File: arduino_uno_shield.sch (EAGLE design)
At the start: 13 parts

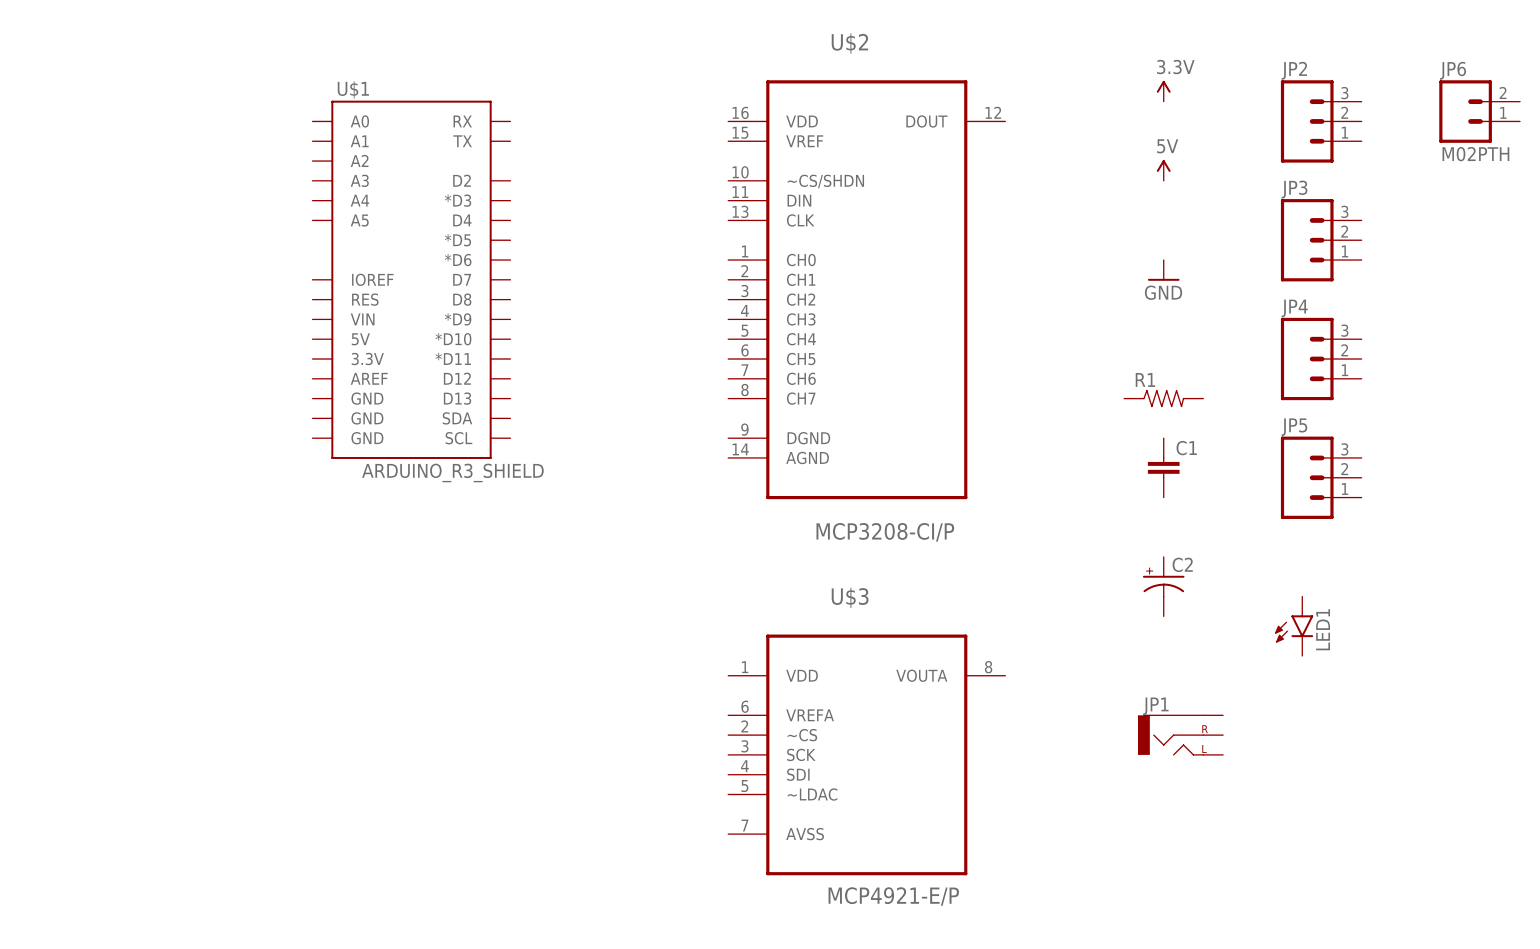
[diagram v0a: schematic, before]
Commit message: wiring up schematic
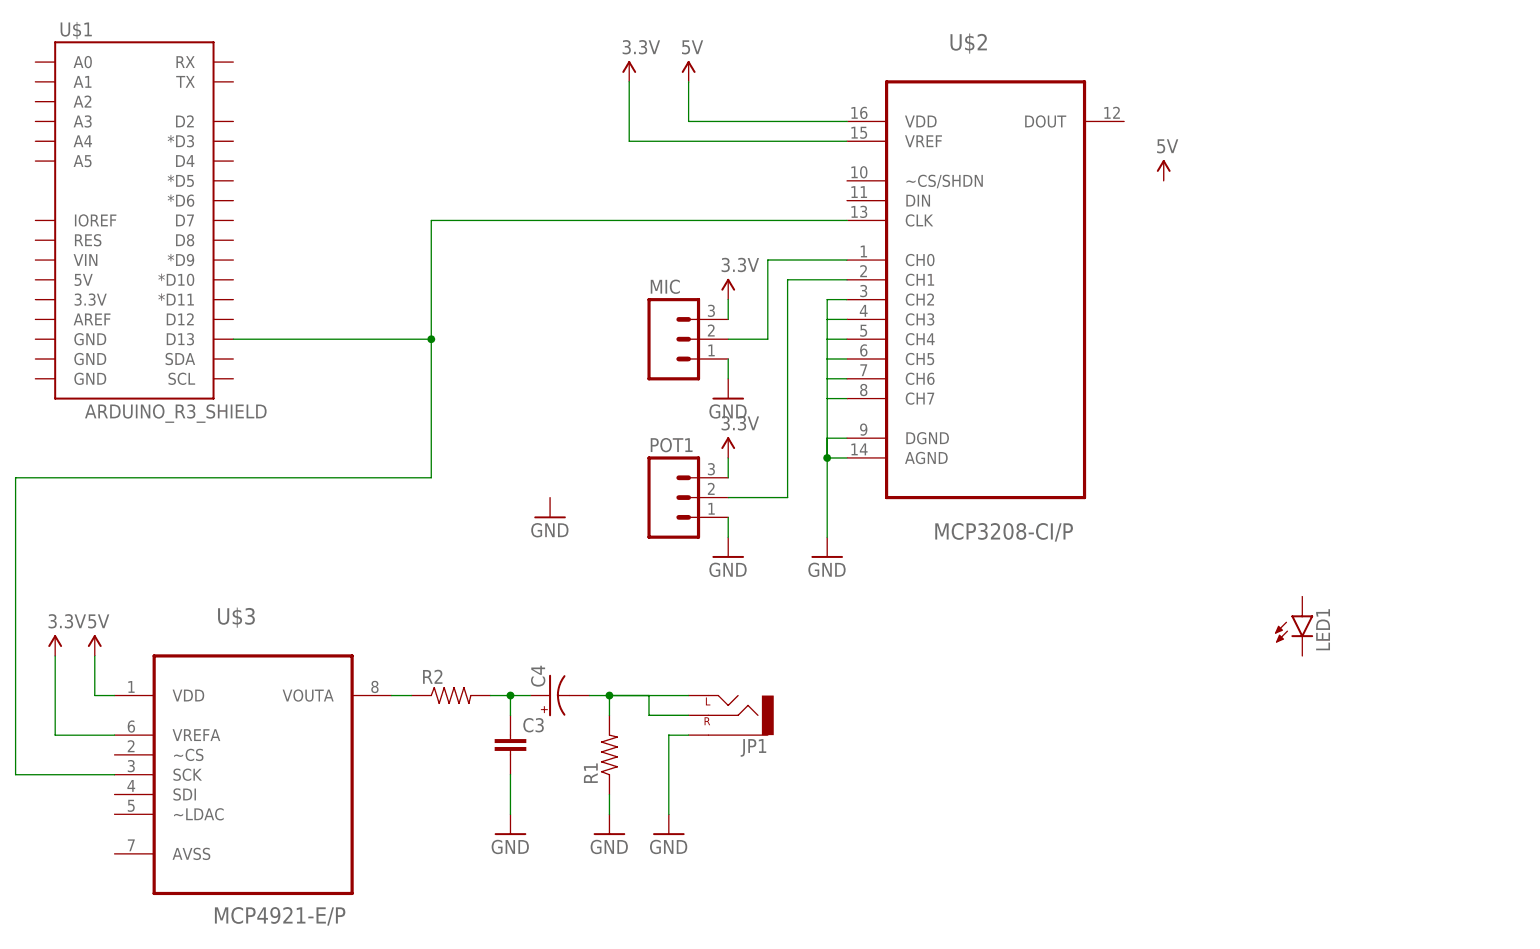
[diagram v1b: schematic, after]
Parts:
- removed C1: (no value), SparkFun-Passives:CAPPTH
- removed C2: (no value), SparkFun-Passives:CAP_POLPTH2
- removed JP2, JP3, JP4, JP5: (no value), SparkFun-Connectors:M03PTH
- removed JP6: M02PTH, SparkFun-Connectors:M02PTH
- added C3: (no value), SparkFun-Passives:CAPPTH
- added C4: (no value), SparkFun-Passives:CAP_POLPTH2
- added MIC, POT1: (no value), SparkFun-Connectors:M03PTH
- added R2: (no value), SparkFun-Passives:RESISTORPTH-1/4W
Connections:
- new net 3.3V: MIC.3, POT1.3, U$2.VREF, U$3.VREFA
- new net 5V: U$2.VDD, U$3.VDD
- new net GND: C3.2, JP1.SLEEVE, MIC.1, POT1.1, R1.1, U$2.AGND, U$2.CH2, U$2.CH3, U$2.CH4, U$2.CH5, U$2.CH6, U$2.CH7, U$2.DGND
- new net N$1: MIC.2, U$2.CH0
- new net N$2: POT1.2, U$2.CH1
- new net N$3: R2.1, U$3.VOUTA
- new net N$4: U$1.D13, U$2.CLK, U$3.SCK
- new net N$8: C3.1, C4.+, R2.2
- new net N$9: C4.-, JP1.LEFT, JP1.RIGHT, R1.2
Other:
- moved on the sheet: JP1, R1, U$1, U$2, U$3
